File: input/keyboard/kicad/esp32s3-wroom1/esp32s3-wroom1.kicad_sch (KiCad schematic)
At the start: 27 parts, among them J1 Conn_01x01_Pin, J10 Conn_01x01_Pin, J11 USB_C_Receptacle_USB2.0_16P, J12 Conn_01x02_Pin, J13 Conn_01x16_Pin, J14 Conn_01x04_Pin, J2 Conn_01x01_Pin, J3 Conn_01x01_Pin, J4 Conn_01x01_Pin, J5 Conn_01x02_Pin, J6 Conn_01x04_Pin, J7 Conn_01x04_Pin, J8 USB_C_Receptacle_USB2.0_16P, J9 Conn_01x01_Pin, U1 ESP32-S3-WROOM-1, U3 TLV1117-33

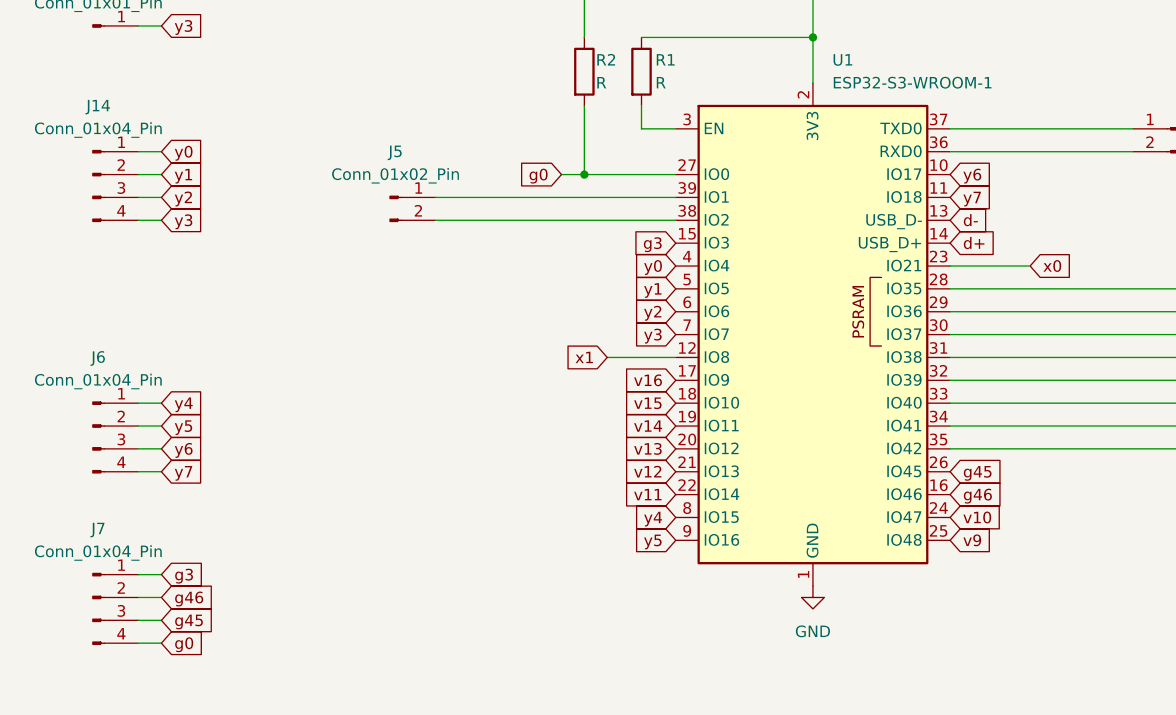
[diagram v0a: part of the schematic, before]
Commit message: input/keyboard: newest working version
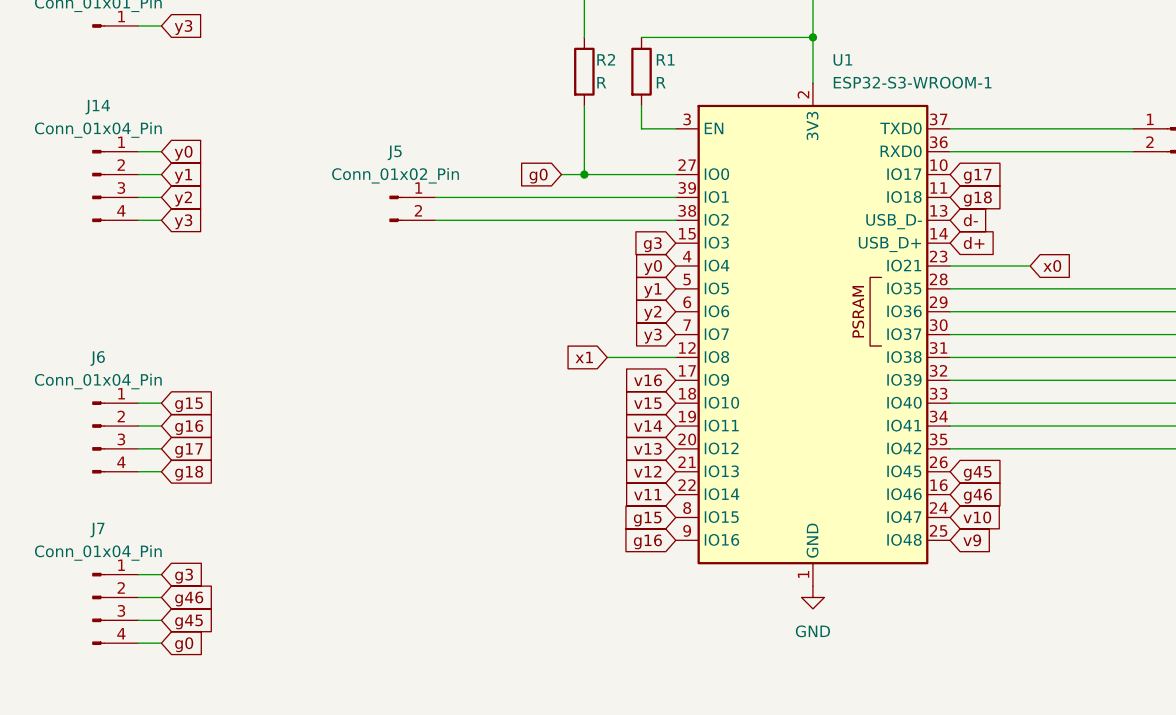
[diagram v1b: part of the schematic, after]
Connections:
- net y4 renamed g15
- net y5 renamed g16
- net y6 renamed g17
- net y7 renamed g18
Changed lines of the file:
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@@
 		)
 	)
-	(global_label "y6"
+	(global_label "g17"
 		(shape input)
 		(at 31.75 87.63 0)
@@
 		)
 		(property "Intersheetrefs" "${INTERSHEET_REFS}"
-			(at 36.9123 87.63 0)
-			(effects
-				(font
-					(size 1.27 1.27)
-				)
-				(justify left)
-				(hide yes)
-			)
-		)
-	)
-	(global_label "y7"
+			(at 38.3032 87.63 0)
+			(effects
+				(font
+					(size 1.27 1.27)
+				)
+				(justify left)
+				(hide yes)
+			)
+		)
+	)
+	(global_label "g18"
 		(shape input)
 		(at 31.75 90.17 0)
@@
 		)
 		(property "Intersheetrefs" "${INTERSHEET_REFS}"
-			(at 36.9123 90.17 0)
+			(at 38.3032 90.17 0)
 			(effects
 				(font
@@
 		)
 	)
-	(global_label "y5"
+	(global_label "g16"
 		(shape input)
 		(at 31.75 85.09 0)
@@
 		)
 		(property "Intersheetrefs" "${INTERSHEET_REFS}"
-			(at 36.9123 85.09 0)
+			(at 38.3032 85.09 0)
 			(effects
 				(font
@@
 		)
 	)
-	(global_label "y4"
+	(global_label "g15"
 		(shape input)
 		(at 31.75 82.55 0)
@@
 		)
 		(property "Intersheetrefs" "${INTERSHEET_REFS}"
-			(at 36.9123 82.55 0)
+			(at 38.3032 82.55 0)
 			(effects
 				(font
@@
 		)
 	)
-	(global_label "y4"
+	(global_label "g15"
 		(shape input)
 		(at 88.9 95.25 180)
@@
 		)
 		(property "Intersheetrefs" "${INTERSHEET_REFS}"
-			(at 83.7377 95.25 0)
+			(at 82.3468 95.25 0)
 			(effects
 				(font
@@
 		)
 	)
-	(global_label "y5"
+	(global_label "g16"
 		(shape input)
 		(at 88.9 97.79 180)
@@
 		)
 		(property "Intersheetrefs" "${INTERSHEET_REFS}"
-			(at 83.7377 97.79 0)
+			(at 82.3468 97.79 0)
 			(effects
 				(font
@@
 		)
 	)
-	(global_label "y7"
+	(global_label "g18"
 		(shape input)
 		(at 119.38 59.69 0)
@@
 		)
 		(property "Intersheetrefs" "${INTERSHEET_REFS}"
-			(at 124.5423 59.69 0)
+			(at 125.9332 59.69 0)
 			(effects
 				(font
@@
 		)
 	)
-	(global_label "y6"
+	(global_label "g17"
 		(shape input)
 		(at 119.38 57.15 0)
@@
 		)
 		(property "Intersheetrefs" "${INTERSHEET_REFS}"
-			(at 124.5423 57.15 0)
-			(effects
-				(font
+			(at 125.9332 57.15 0)
+			(effects
+				(font
